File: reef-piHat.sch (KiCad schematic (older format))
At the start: 33 parts, among them J1 Doser, J10 ATO2, J11 ph1, J12 ph2, J13 5vPower, J14 Temp1, J15 Temp2, J16 Temp3, J2 Light1, J3 40HAT, J4 Light2, J5 12vPower, J6 Power2, J7 Power1, J8 ATO1, Q1 DMMT5401, Q2 DMG2305UX, U1 PCA9685PW, U2 CAT24C32, U3 ULN2803A

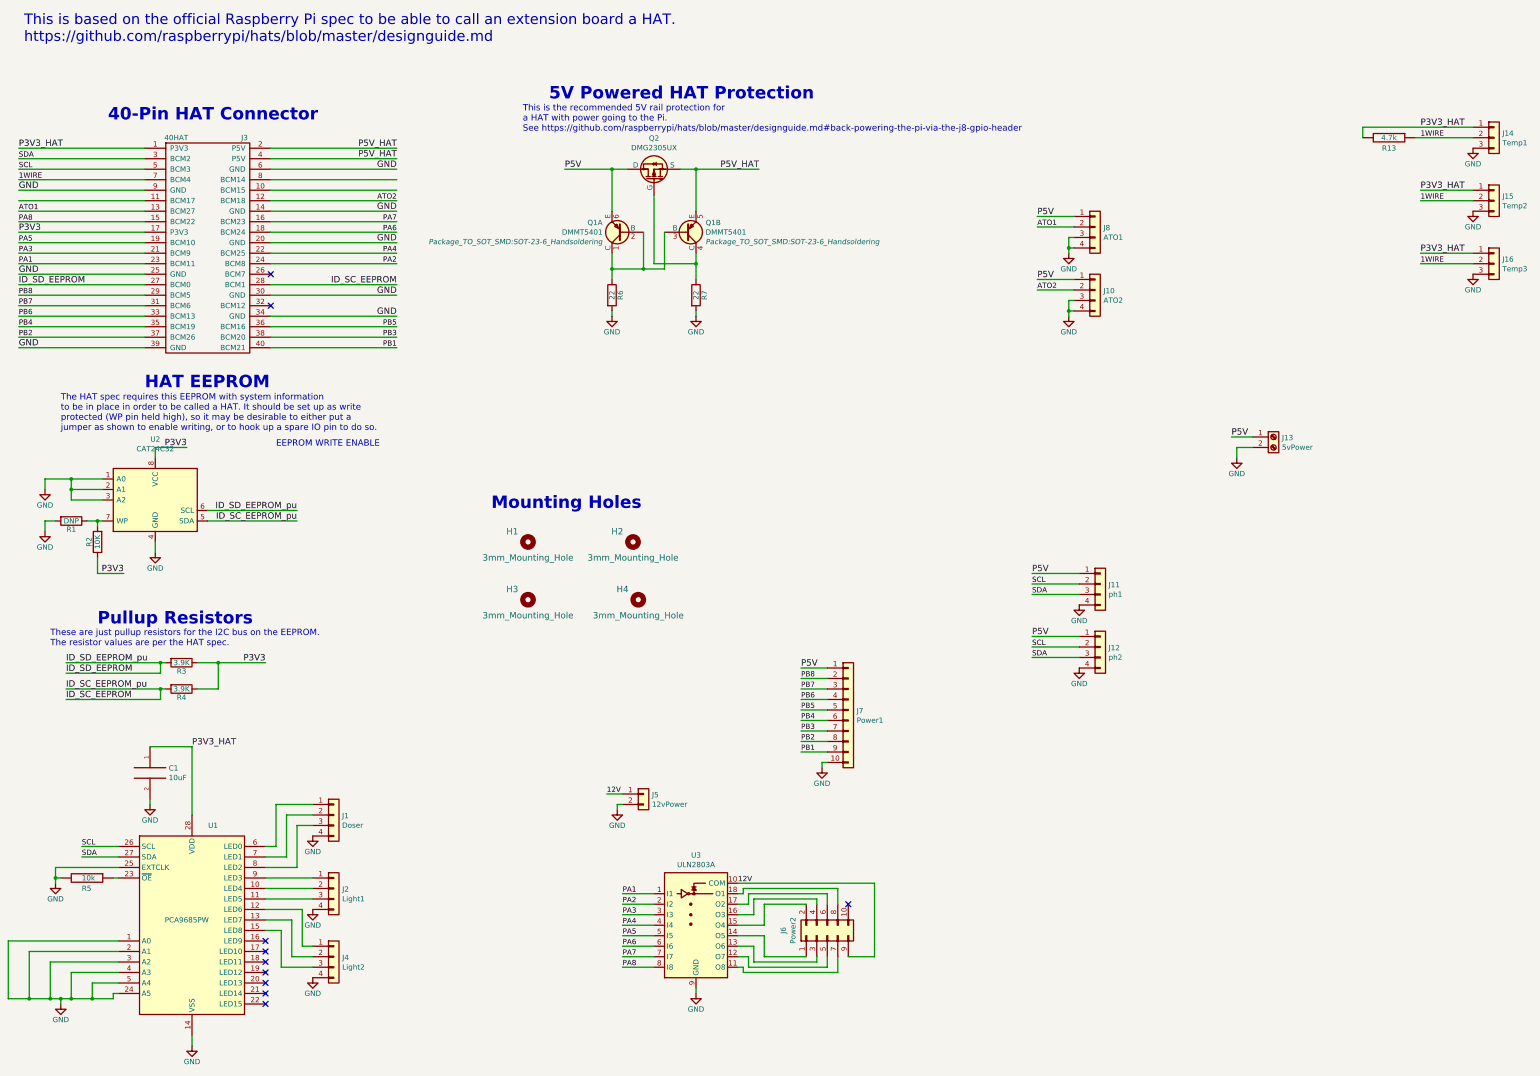
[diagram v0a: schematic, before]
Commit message: Add readme and images
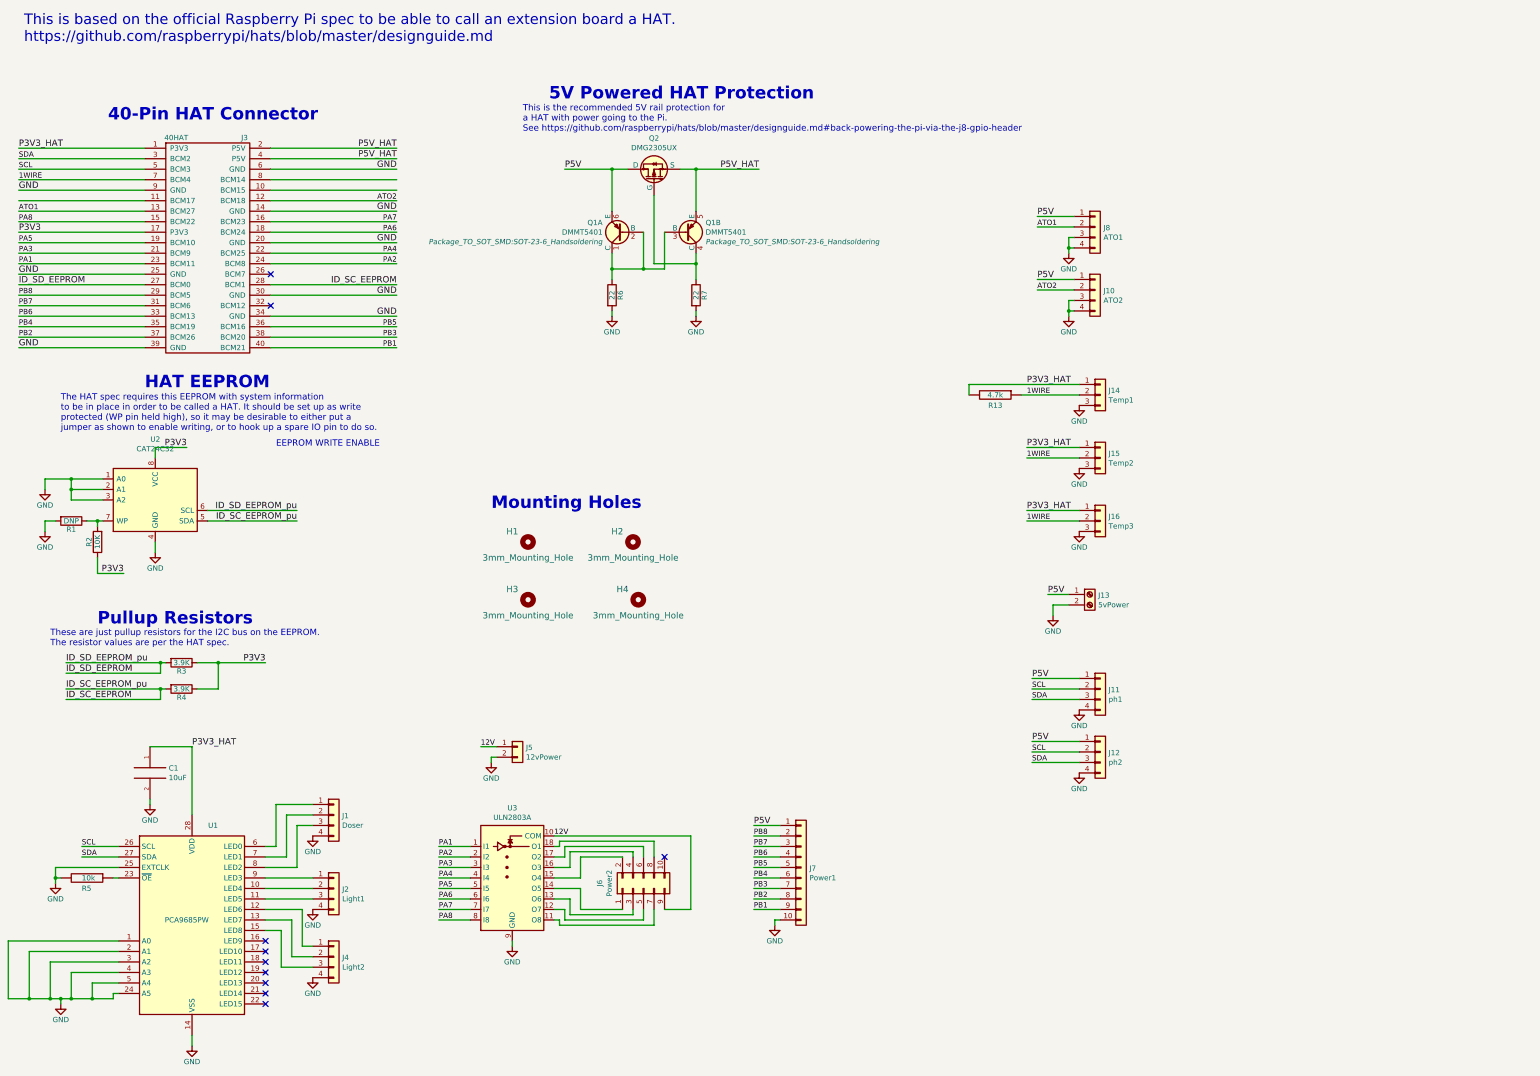
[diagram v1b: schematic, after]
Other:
- moved on the sheet: J11, J12, J13, J14, J15, J16, J5, J6, J7, R13, U3
